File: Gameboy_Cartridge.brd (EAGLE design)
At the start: 49.3 x 48 mm, 10 parts, among them IC1 AT49F040J

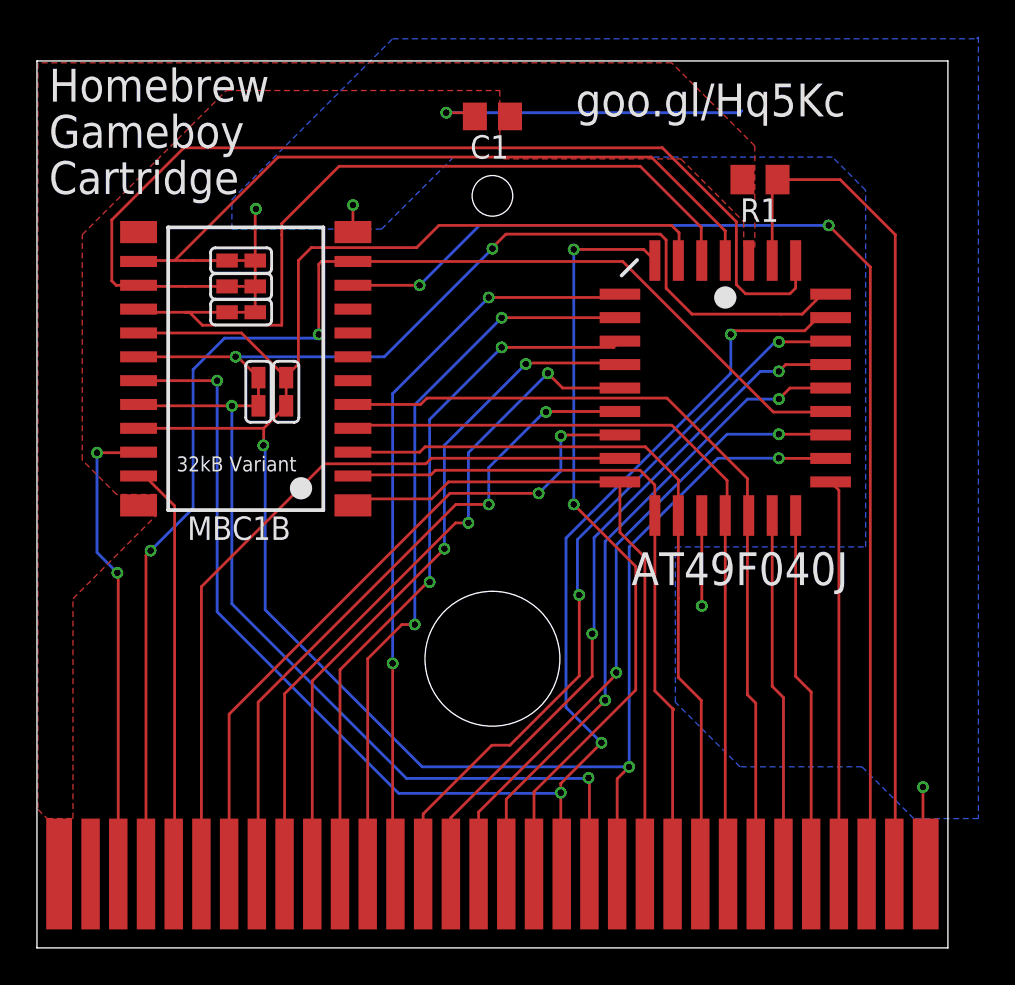
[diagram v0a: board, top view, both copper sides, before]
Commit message: Other changes to make it prettier
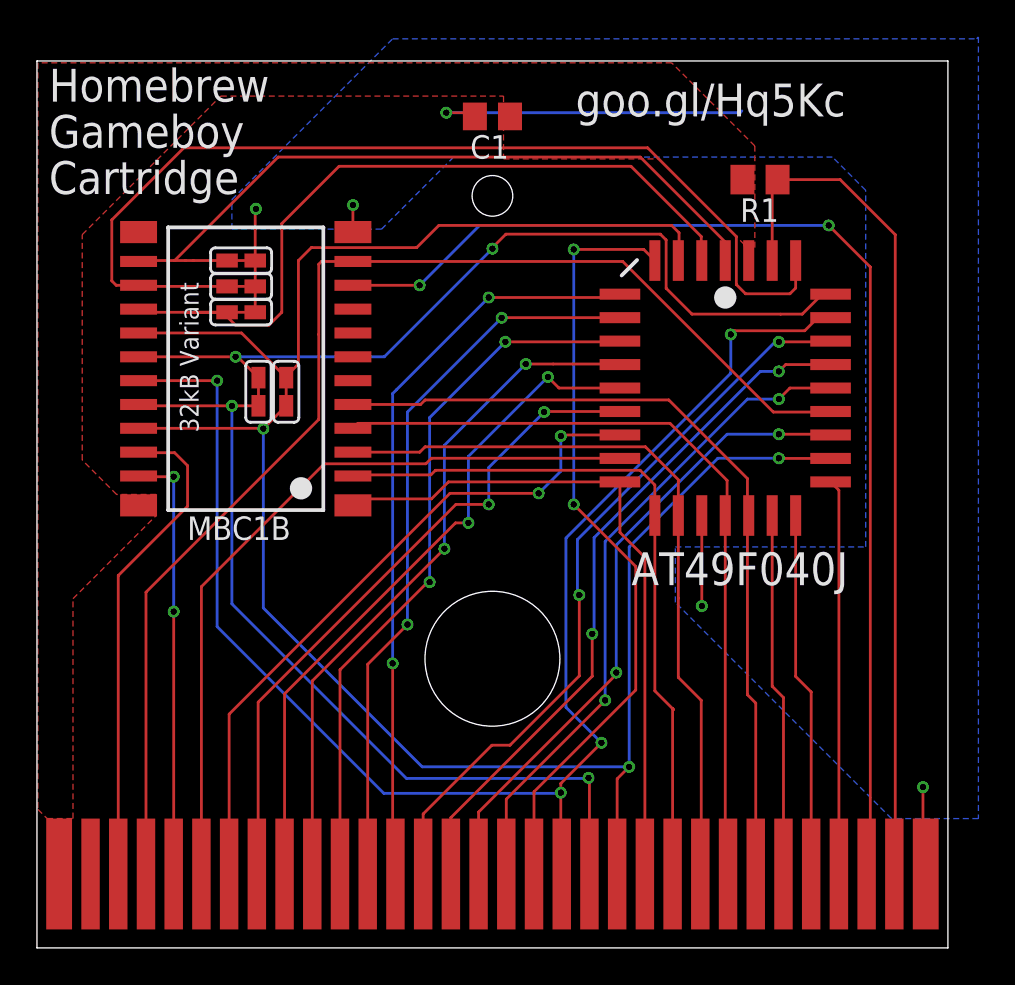
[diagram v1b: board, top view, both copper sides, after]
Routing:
- net 4: track 71.2 -> 68.3 mm, vias 2 -> 0
- net 3: track 25.5 -> 26.7 mm, vias 2 -> 0
- net 5: track 22.6 -> 23.4 mm, vias 0 -> 2
- net C: track 43.1 -> 42.4 mm
